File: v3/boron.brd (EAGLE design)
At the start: 100 x 80 mm, 47 parts, among them J1 batt, J10 USB_MINI-B_SMT, J11 drv, J12 out, J13 RASM722, J14 debug, J16 5V, J4 ISP, Q1 Si7137DP, U2_C1 10nF, U2_C2 2.2uF, U2_L1 1 kOhm @ 100MHz, U2_L2 1 kOhm @ 100MHz, U2_R1 10k, U2_R2 10k, U2_R9 100K Ohms, U3 ATTINY84-20MU, U6 TPS61230A, U6_CBST 10 nF, U6_CFF 10pF, U6_CIN 22uF, U6_COUT 22uF, U6_RFBB 100K Ohms, U6_RFBT 316K Ohms, U9 BQ24168RGET

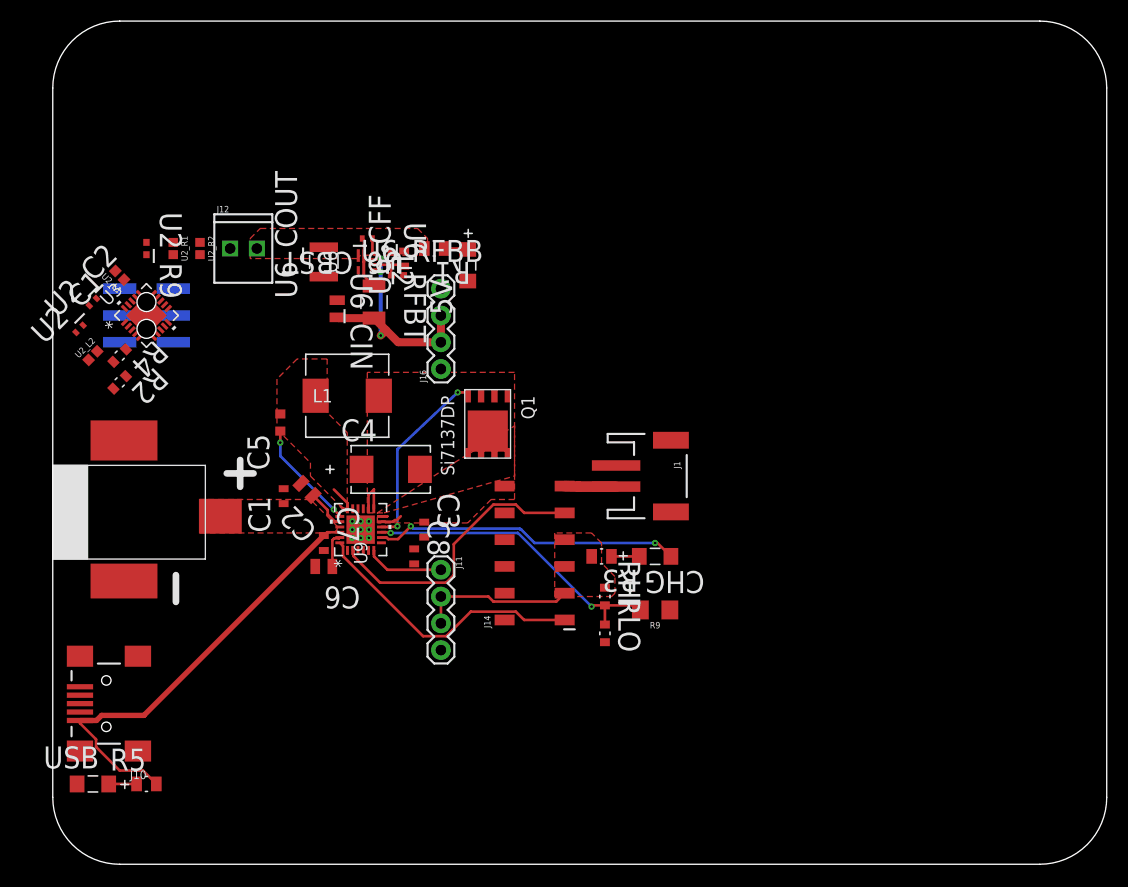
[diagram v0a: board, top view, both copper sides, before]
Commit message: Boron off to OSH.
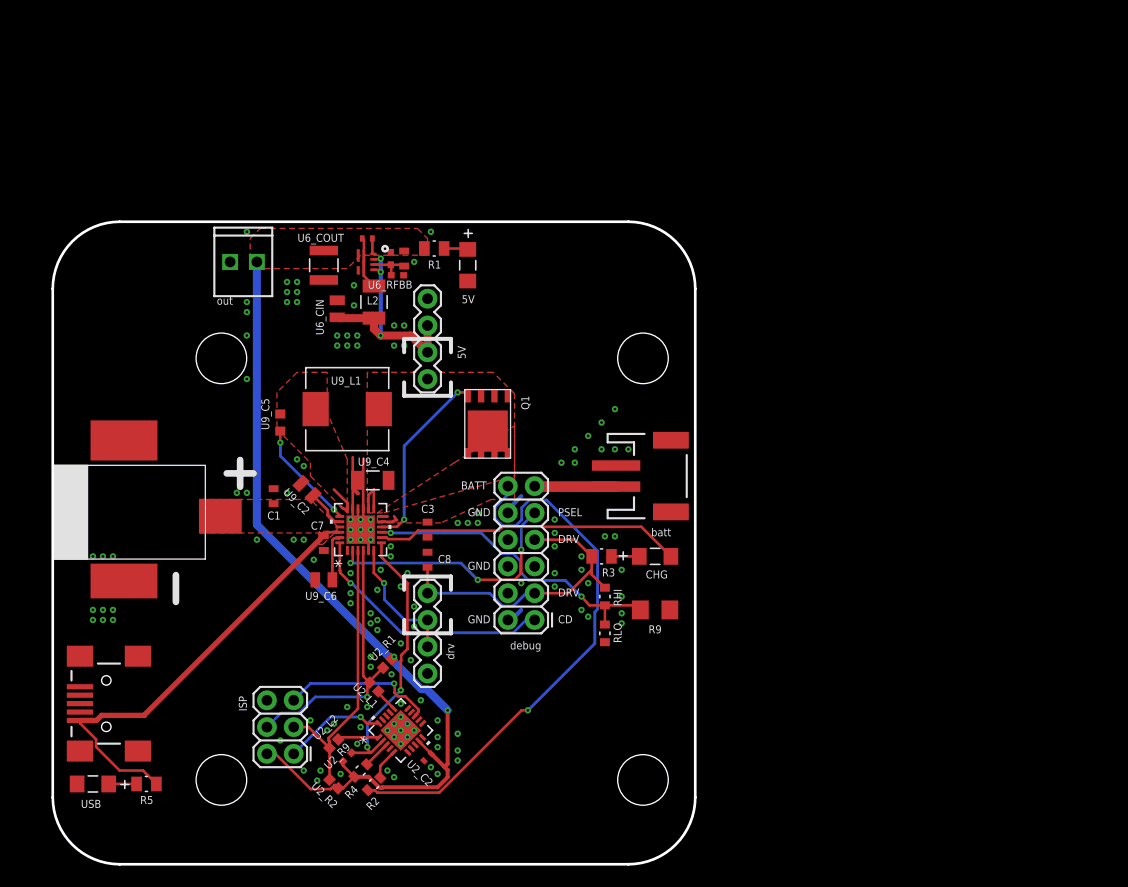
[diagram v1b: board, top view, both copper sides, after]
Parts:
- removed C4: 47UF, AVX_By_element14_Batch_1:CAPCP7343X430N
- removed C6: 4.7uF, AVX_By_element14_Batch_1:CAPC2013X140N
- removed L1: DR73-2R2-R, 32bits:DR73
- removed U2_C1: 10nF, Yageo_By_element14_Batch_1:CAPC1005X55N
- added U9_C4: 47uF, AVX_By_element14_Batch_1:CAPC3216X127N
- added U9_C6: 4.7uF, AVX_By_element14_Batch_1:CAPC2013X140N
- added U9_L1: DR73-2R2-R, 32bits:DR73
- J14: device SparkFun-Connectors:2X6_SMD -> SparkFun-Connectors:2X6
- J4: device SparkFun-Connectors:2X3_SMT_POSTS -> SparkFun-Connectors:2X3
- moved U2_C2 53.6 mm to (35.6, 10.2)
- moved U2_R2 52.4 mm to (26.7, 7.62), turned to 135 degrees
- moved U2_R9 51.9 mm to (27.9, 10.2), turned to 45 degrees
- moved U3 46.2 mm to (33.0, 12.7)
- moved U2_L1 45.9 mm to (30.5, 16.8)
- moved R4 45.5 mm to (29.2, 8.89)
- moved R2 45.1 mm to (30.5, 7.62)
- moved U2_R1 44.3 mm to (31.8, 19.1), turned to 225 degrees
- moved J4 43.9 mm to (22.9, 10.5), flipped to the top
- moved U2_L2 43.3 mm to (26.7, 11.4)
- moved J14 6.35 mm to (45.7, 23.2)
- moved 5 4.80 mm to (44.7, 5.08)
- moved J11 2.56 mm to (35.6, 25.7)
- moved J16 1.59 mm to (35.6, 46.0)
- moved C8 1.31 mm to (35.6, 28.9)
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- renumbered C2 to U9_C2, C5 to U9_C5
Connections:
- removed net U9_DRV_O: C8.2, J11.1, U9.6
- new net U9_DRV_0: J11.2, J11.3, U9.6
- net GND: now also U3.21, U9_C4.1, U9_C6.2; no longer C4.1, C6.2, U2_C1.1
- net SYS_5V: no longer U2_C1.2
- net U9_DRV: now also C8.2, J11.1; no longer J11.2, J11.3
- net U9_PMIDU: now also U9_C6.1; no longer C6.1
- net U9_SW: now also U9_L1.1; no longer L1.1
- net U9_SYS: now also U9_C4.2, U9_L1.2; no longer C4.2, L1.2
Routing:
- net SYS_5V: track 0.00 -> 83.8 mm, vias 0 -> 2
- net VBAT: track 2.62 -> 56.2 mm, vias 0 -> 1
- net U9_SCL: track 0.00 -> 27.2 mm
- net U9_SDA: track 0.00 -> 26.9 mm, vias 0 -> 1
- net U9_INT: track 0.00 -> 26.1 mm, vias 0 -> 2
- net GND: track 0.00 -> 18.9 mm, vias 0 -> 135
- net !RESET: track 0.00 -> 14.7 mm, vias 0 -> 1
- net U9_DRV: track 14.8 -> 29.5 mm
- net U9_DRV_0: track 0.00 -> 12.5 mm, vias 0 -> 1
- net MISO: track 0.00 -> 9.79 mm, vias 0 -> 1
- net U9_DRV_O: track 7.45 -> 0.00 mm
- net U3_PA4: track 0.00 -> 3.95 mm
- net ADC0: track 0.00 -> 2.95 mm
- net VBAT_CON: track 4.88 -> 7.75 mm
- net U9_CD: track 26.9 -> 24.2 mm, vias 0 -> 1
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- added copper zone on layer 1, net GND
- added copper zone on layer 16, net GND
- added copper zone on layer 1, net U9_USB
- removed copper zone on layer 1, net U9_DRV
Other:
- board size 100 x 80 mm -> 61 x 61 mm
- board text added: "BATT"
- board text added: "CD"
- board text added: "DRV"
- board text added: "GND"
- board text added: "PSEL"
